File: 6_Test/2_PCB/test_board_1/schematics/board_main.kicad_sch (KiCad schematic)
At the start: 29 parts, among them J1 Digital_Outputs, J10 Analog_Inputs_Jumpers, J3 BNC1, J4 Digital_Inputs, J5 BNC_to_Analog, J6 BNC2, J7 Conn_02x06_Row_Letter_First, J8 IOVDD_Jumpers, J9 Power_Connector

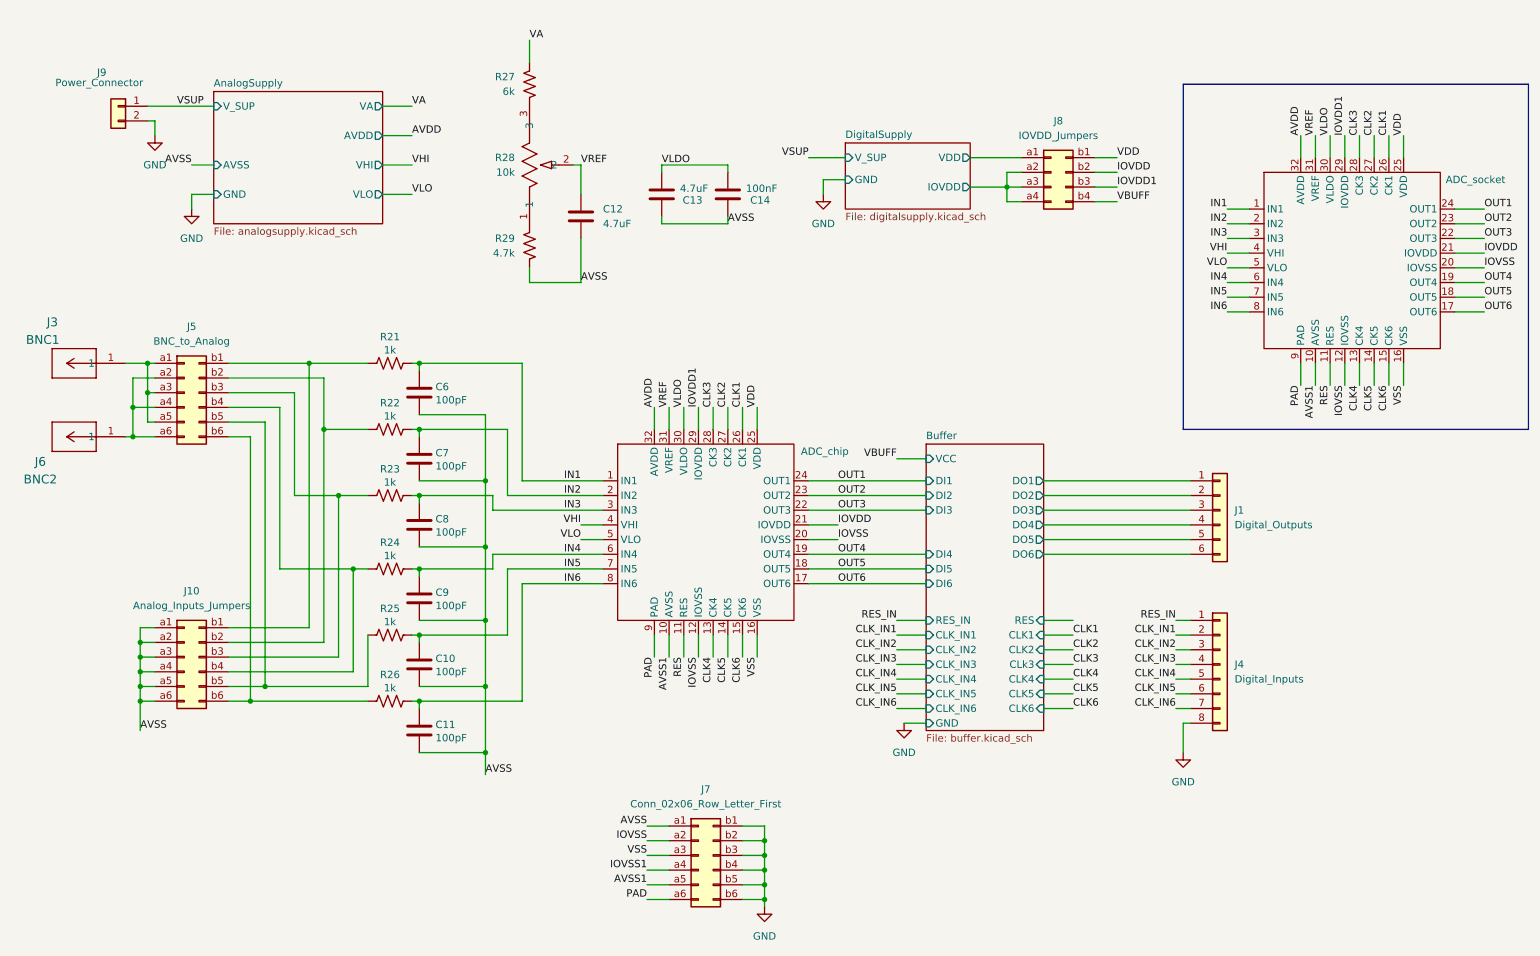
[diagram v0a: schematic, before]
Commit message: creating new project. combining work
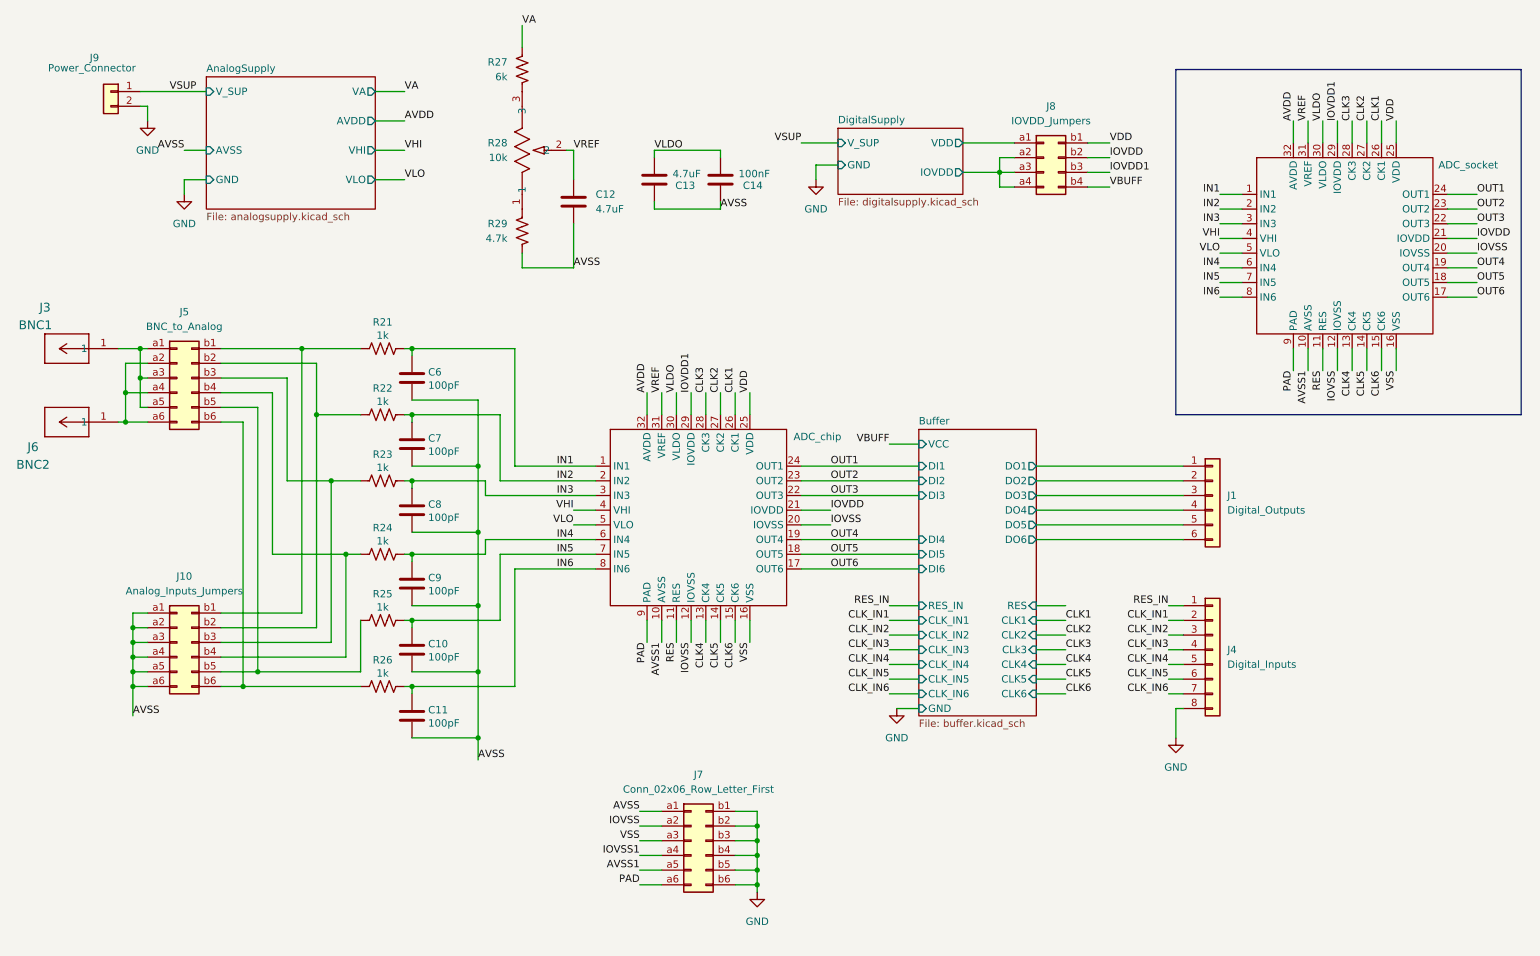
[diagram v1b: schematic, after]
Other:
- moved on the sheet: ADC_chip, ADC_socket, C10, C11, C12, C13, C14, C6, C7, C8, C9, J1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
